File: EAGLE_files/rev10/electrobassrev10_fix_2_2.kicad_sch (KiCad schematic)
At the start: 22 parts, among them U14 CY8C4024AZI-S413TQFP_24AZI-S4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

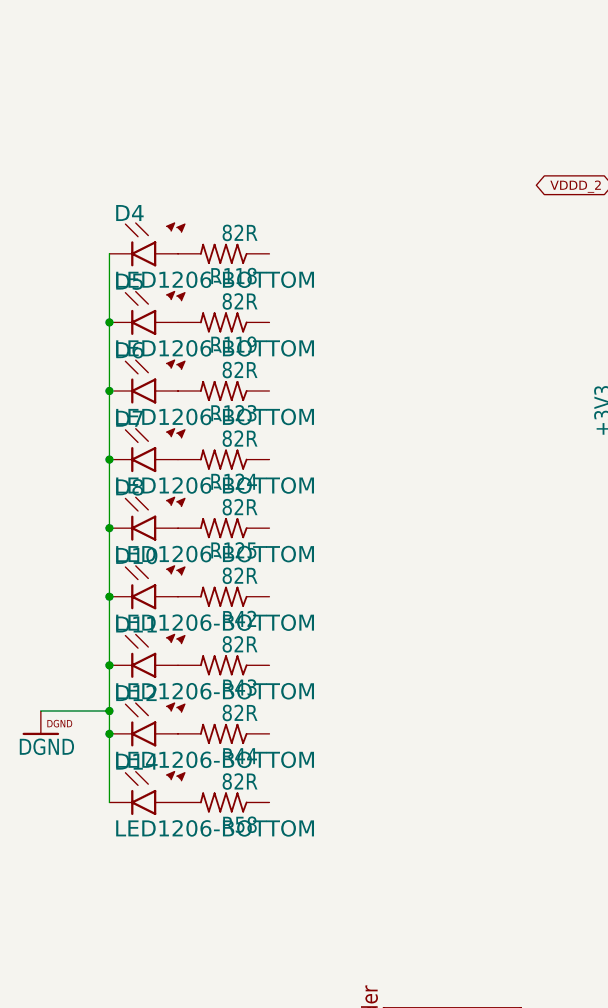
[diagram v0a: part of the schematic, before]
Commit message: added new electrobass revision kicad files
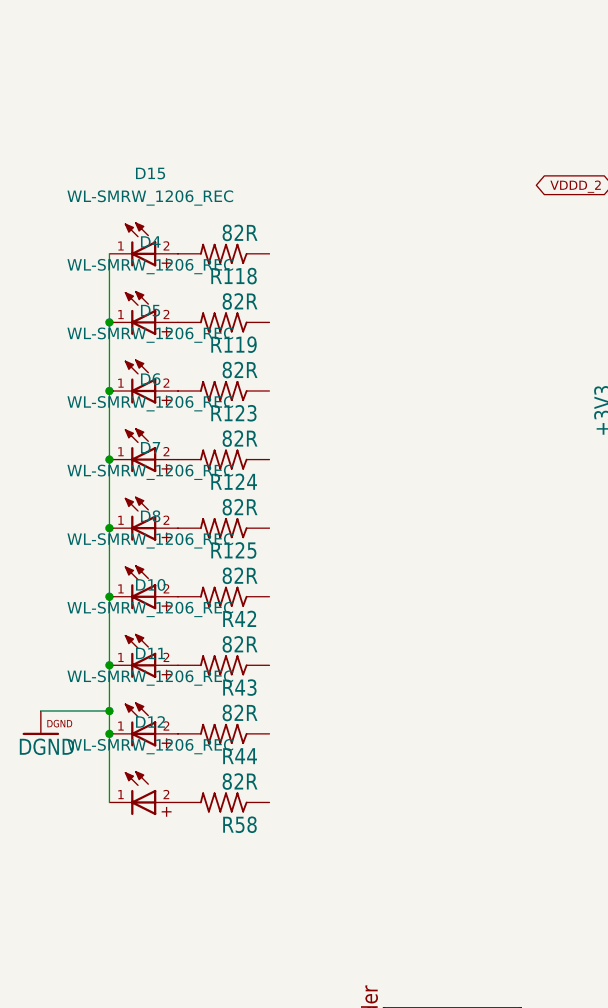
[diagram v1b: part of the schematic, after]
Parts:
- removed D10, D11, D12, D14, D4, D5, D6, D7, D8: LED1206-BOTTOM, electrobassrev10_fix_2:LED-1206-BOTTOM, symbol electrobassrev10_fix_2-eagle-import:LED1206-BOTTOM
- added D10, D11, D12, D15, D4, D5, D6, D7, D8: WL-SMRW_1206_REC, Snapeda:WL-SMRW_1206_REC, symbol Snapeda:WL-SMRW_1206_REC
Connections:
- net DGND: now also D10.1, D11.1, D12.1, D15.1, D4.1, D5.1, D6.1, D7.1, D8.1
- net at R42.2: now also D8.2
- net at R123.2: now also D5.2
- net at R125.2: now also D7.2
- net at R119.2: now also D4.2
- net at R58.2: now also D12.2
- net at R44.2: now also D11.2
- net at R118.2: now also D15.2
- net at R43.2: now also D10.2
- net at R124.2: now also D6.2
